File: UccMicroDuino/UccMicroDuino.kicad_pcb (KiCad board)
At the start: 2 copper layers, 8 x 7.5 mm, 8 parts, among them J1 Conn_01x10_Socket, J2 USB_A, U1 ATtiny85-20S

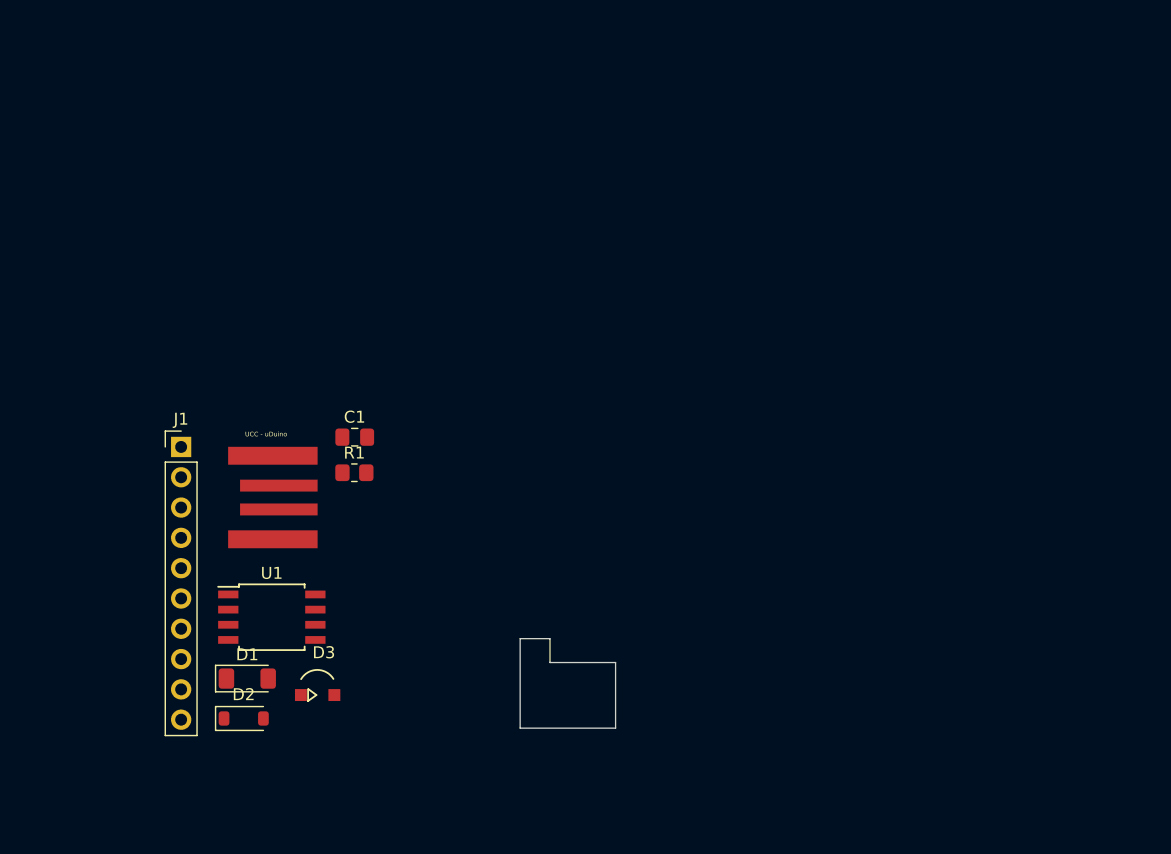
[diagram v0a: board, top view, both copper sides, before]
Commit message: clase 5 de mayo
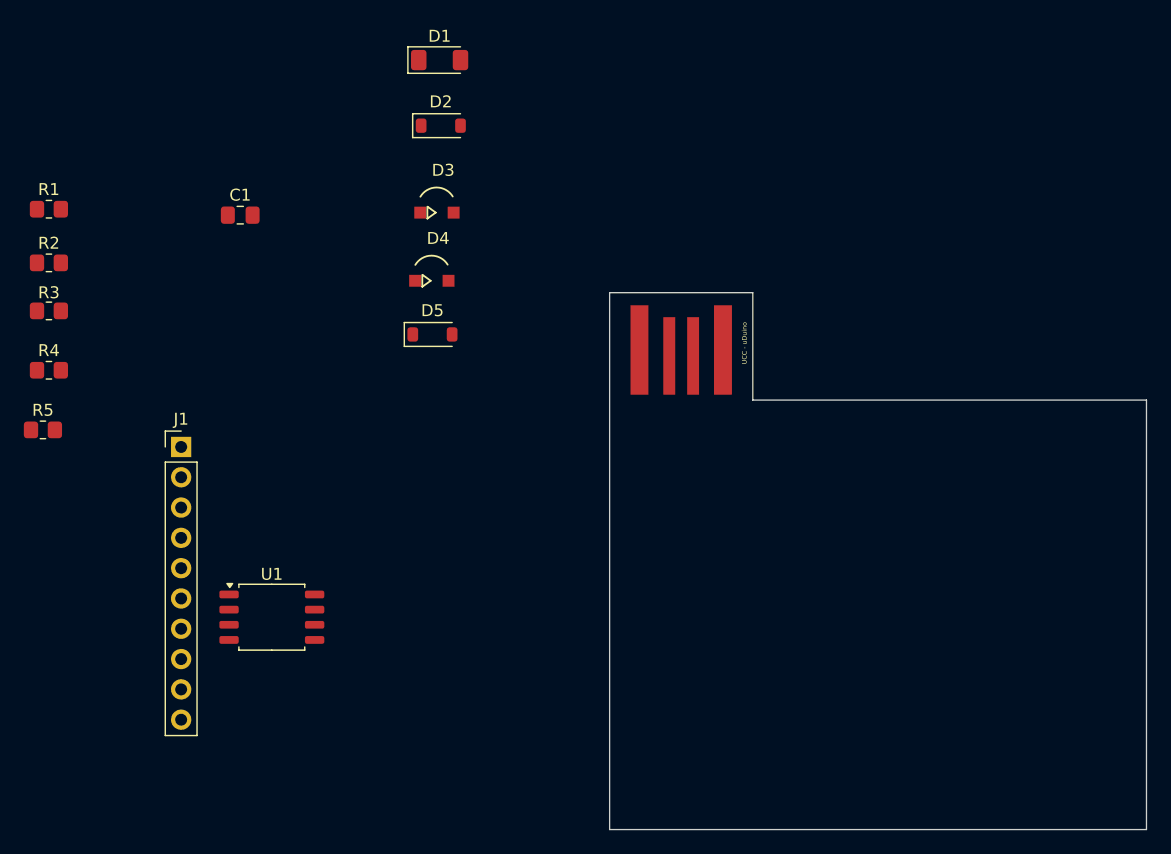
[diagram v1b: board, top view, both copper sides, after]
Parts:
- added D4: LED GREEN, ledSmd:ledSMD, F.Cu at (145.5, 54.0)
- added D5: 3.6 V 1/2 W, Diode_SMD:D_SOD-123, F.Cu at (145.2, 58.5)
- added R2: 300 omhs 5% 1/8w, Resistor_SMD:R_0805_2012Metric_Pad1.20x1.40mm_HandSolder, F.Cu at (113.0, 52.5)
- added R3: 68 omhs 5% 1/8w, Resistor_SMD:R_0805_2012Metric_Pad1.20x1.40mm_HandSolder, F.Cu at (113.0, 56.5)
- added R4: 68 omhs 5% 1/8w, Resistor_SMD:R_0805_2012Metric_Pad1.20x1.40mm_HandSolder, F.Cu at (113.0, 61.5)
- added R5: 300 omhs 5% 1/8w, Resistor_SMD:R_0805_2012Metric_Pad1.20x1.40mm_HandSolder, F.Cu at (112.5, 66.5)
- C1: value C -> 0.1u
- D2: value D_Zener -> 3.6 V 1/2 W
- D3: value LED -> LED RED
- R1: value R -> 1.5 omhs 5% 1/8w
- U1: footprint Package_SO:SOIC-8W_5.3x5.3mm_P1.27mm -> Package_SO:SOIC-8_5.3x5.3mm_P1.27mm
- moved D1 54.3 mm to (145.8, 35.5)
- moved D2 52.4 mm to (145.8, 41.0)
- moved D3 41.7 mm to (145.9, 48.3)
- moved J2 36.1 mm to (166.0, 60.0), turned to -90 degrees
- moved R1 33.8 mm to (113.0, 48.0)
- moved C1 20.9 mm to (129.0, 48.5)
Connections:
- C1 pad 1: unconnected-(C1-Pad1) -> +5V
- C1 pad 2: unconnected-(C1-Pad2) -> GND
- D1 pad 2: unconnected-(D1-A-Pad2) -> Net-(D1-A)
- D2 pad 1: unconnected-(D2-K-Pad1) -> Net-(D2-K)
- D2 pad 2: unconnected-(D2-A-Pad2) -> GND
- D3 pad 1: unconnected-(D3-K-Pad1) -> Net-(D3-K)
- D3 pad 2: unconnected-(D3-A-Pad2) -> +5V
- J1 pad 1: unconnected-(J1-Pin_1-Pad1) -> +5V
- J1 pad 2: unconnected-(J1-Pin_2-Pad2) -> GND
- J1 pad 4: unconnected-(J1-Pin_4-Pad4) -> Net-(J1-Pin_4)
- J1 pad 5: unconnected-(J1-Pin_5-Pad5) -> Net-(D4-A)
- J1 pad 6: unconnected-(J1-Pin_6-Pad6) -> Net-(J1-Pin_6)
- J1 pad 7: unconnected-(J1-Pin_7-Pad7) -> Net-(J1-Pin_7)
- J1 pad 8: unconnected-(J1-Pin_8-Pad8) -> Net-(J1-Pin_8)
- J1 pad 9: unconnected-(J1-Pin_9-Pad9) -> Net-(J1-Pin_9)
- J2 pad 1: unconnected-(J2-VBUS-Pad1) -> Net-(D1-A)
- J2 pad 2: unconnected-(J2-D--Pad2) -> Net-(D2-K)
- J2 pad 3: unconnected-(J2-D+-Pad3) -> Net-(D5-K)
- J2 pad 4: unconnected-(J2-GND-Pad4) -> GND
- R1 pad 2: unconnected-(R1-Pad2) -> Net-(D2-K)
- U1 pad 1: unconnected-(U1-~{RESET}/PB5-Pad1) -> Net-(J1-Pin_9)
- U1 pad 2: unconnected-(U1-XTAL1/PB3-Pad2) -> Net-(J1-Pin_7)
- U1 pad 3: unconnected-(U1-XTAL2/PB4-Pad3) -> Net-(J1-Pin_8)
- U1 pad 4: unconnected-(U1-GND-Pad4) -> GND
- U1 pad 5: unconnected-(U1-AREF/PB0-Pad5) -> Net-(J1-Pin_4)
- U1 pad 6: unconnected-(U1-PB1-Pad6) -> Net-(D4-A)
- U1 pad 7: unconnected-(U1-PB2-Pad7) -> Net-(J1-Pin_6)
- U1 pad 8: unconnected-(U1-VCC-Pad8) -> +5V
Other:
- board size 8 x 7.5 mm -> 45 x 45 mm
